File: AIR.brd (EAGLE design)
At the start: 100 x 47 mm, 32 parts

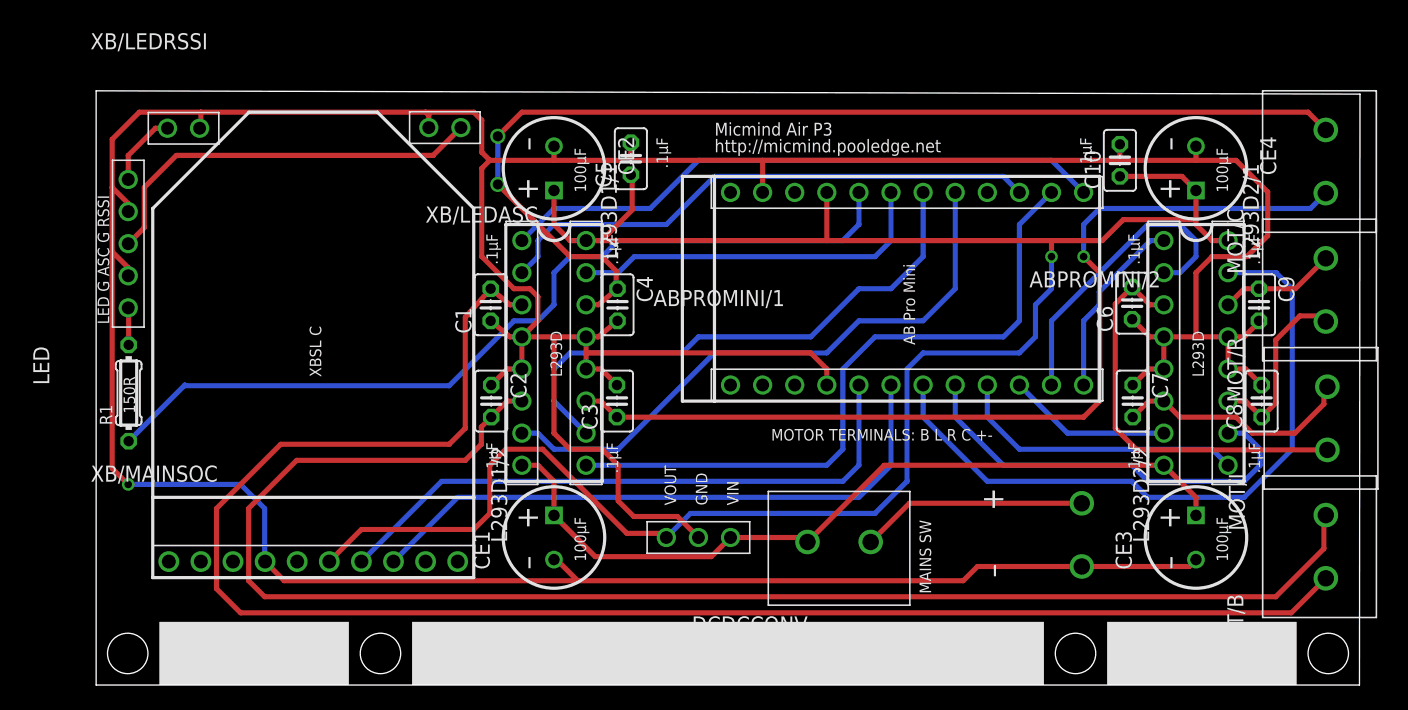
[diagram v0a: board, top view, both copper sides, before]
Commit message: Major improvements on hardware, patch stability
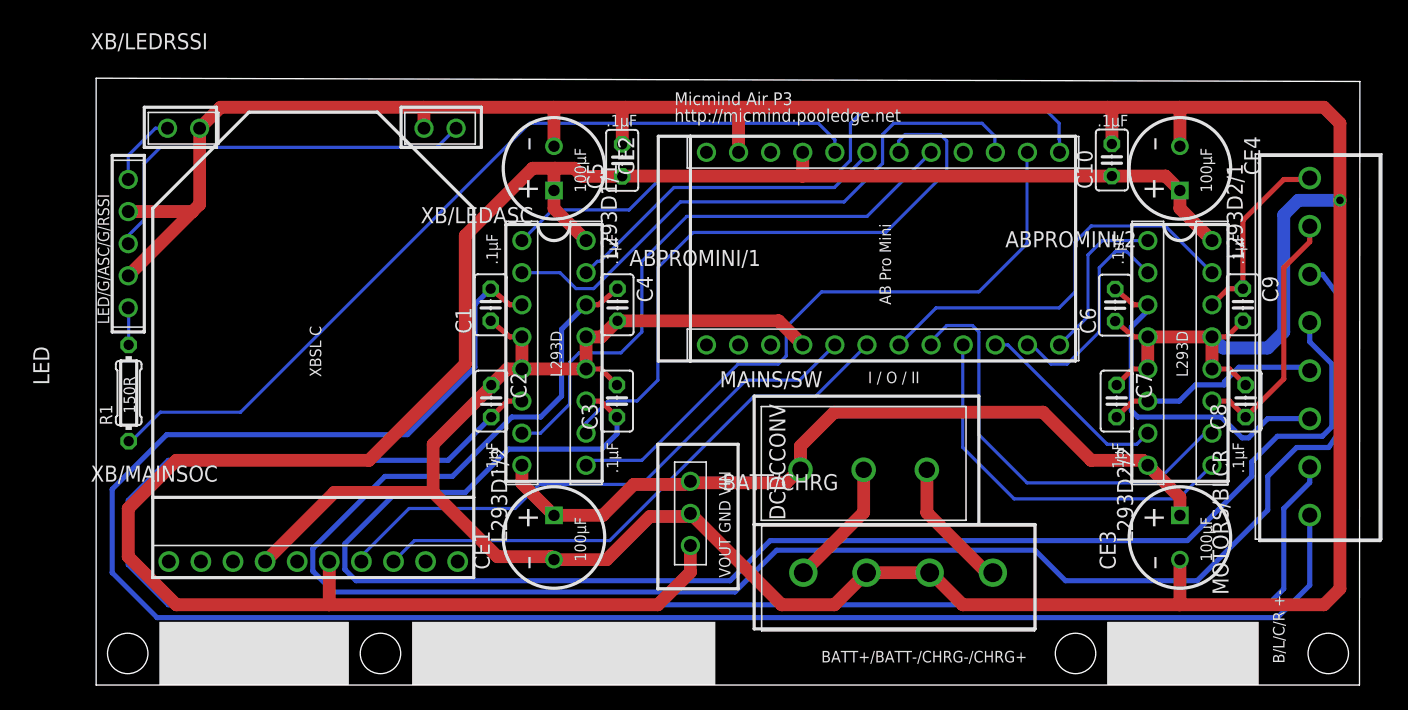
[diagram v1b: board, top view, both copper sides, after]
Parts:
- removed MAINS/BATT, MOT/B, MOT/C, MOT/L, MOT/R: 691101710002, Wurth_Elektronik_Electromechanic_Terminal_Blocks_Connectors_rev15b:691101710002
- added BATT/CHRG: 691121710004, Wurth_Elektronik_Electromechanic_Terminal_Blocks_Connectors_rev15b:691121710004
- added MOTORS/BLCR: 691221320008, Wurth_Elektronik_Electromechanic_Terminal_Blocks_Connectors_rev15b:691221320008
- MAINS/SW: value 691101710002 -> 691101710003; device Wurth_Elektronik_Electromechanic_Terminal_Blocks_Connectors_rev15b:691101710002 -> Wurth_Elektronik_Electromechanic_Terminal_Blocks_Connectors_rev15b:691101710003
- moved MAINS/SW 7.24 mm to (60.7, 17.0), turned to 0 degrees
- moved ABPROMINI/2 3.70 mm to (62.3, 42.2)
- moved ABPROMINI/1 3.70 mm to (62.3, 26.9)
- moved DCDCCONV 2.01 mm to (47.0, 13.6), turned to 270 degrees
- moved C6 1.35 mm to (80.6, 30.1)
- moved C7 1.27 mm to (80.8, 22.5)
- moved C8 1.27 mm to (91.0, 22.5)
- moved C9 1.27 mm to (90.7, 30.1)
- moved CE3 1.27 mm to (85.8, 11.7)
- moved CE4 1.27 mm to (85.8, 40.9)
- moved L293D2/1 1.27 mm to (83.2, 26.3)
- moved L293D2/2 1.27 mm to (88.3, 26.3)
- moved C5 0.70 mm to (41.6, 41.5)
- moved C10 0.64 mm to (80.4, 41.5)
- moved XB/LEDASC 0.38 mm to (27.2, 44.1)
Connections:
- new net N$4: BATT/CHRG.4, MAINS/SW.3
- net +24V: now also MAINS/SW.1; no longer MAINS/SW.2
- net GND: now also BATT/CHRG.2, BATT/CHRG.3; no longer MAINS/BATT.2
- net MB+: now also MOTORS/BLCR.1; no longer MOT/B.1
- net MB-: now also MOTORS/BLCR.2; no longer MOT/B.2
- net MC+: now also MOTORS/BLCR.5; no longer MOT/C.1
- net MC-: now also MOTORS/BLCR.6; no longer MOT/C.2
- net ML+: now also MOTORS/BLCR.3; no longer MOT/L.1
- net ML-: now also MOTORS/BLCR.4; no longer MOT/L.2
- net MR+: now also MOTORS/BLCR.7; no longer MOT/R.1
- net MR-: now also MOTORS/BLCR.8; no longer MOT/R.2
- net N$3: now also BATT/CHRG.1, MAINS/SW.2; no longer MAINS/BATT.1, MAINS/SW.1
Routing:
- net MC-: track 87.3 -> 142.3 mm, vias 2 -> 0
- net MC+: track 76.4 -> 124.6 mm, vias 1 -> 0
- net D4: track 54.3 -> 32.5 mm
- net MB-: track 121.6 -> 143.3 mm
- net MB+: track 133.1 -> 151.8 mm
- net N$4: track 0.00 -> 10.6 mm
- net +5V: track 162.9 -> 171.3 mm, vias 1 -> 0
- net N$3: track 18.0 -> 10.1 mm
- net D6~: track 23.2 -> 30.6 mm
- net D8: track 24.5 -> 17.5 mm
- net A1: track 44.1 -> 50.4 mm
- net MR+: track 14.7 -> 20.4 mm
- net MR-: track 9.26 -> 14.9 mm
- net ML+: track 32.3 -> 27.6 mm
- net D3: track 48.9 -> 44.6 mm
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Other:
- board size 100 x 47 mm -> 100 x 48 mm
- board text added: "B/L/C/R +-"
- board text added: "BATT+/BATT-/CHRG-/CHRG+"
- board text added: "I / O / II"
- board text added: "LED/G/ASC/G/RSSI"
- board text removed: "LED G ASC G RSSI"
- board text removed: "MAINS SW"
- board text removed: "MOTOR TERMINALS: B L R C +-"
